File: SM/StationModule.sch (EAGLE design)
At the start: 25 parts, among them IC1 REG1117

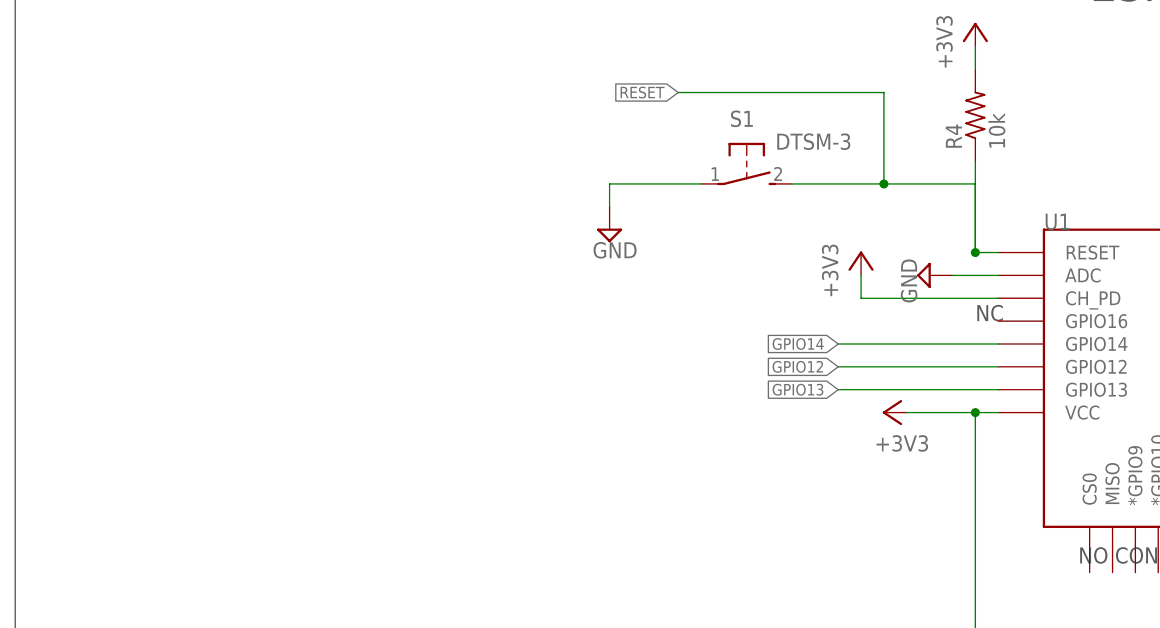
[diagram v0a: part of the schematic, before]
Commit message: silkscreen
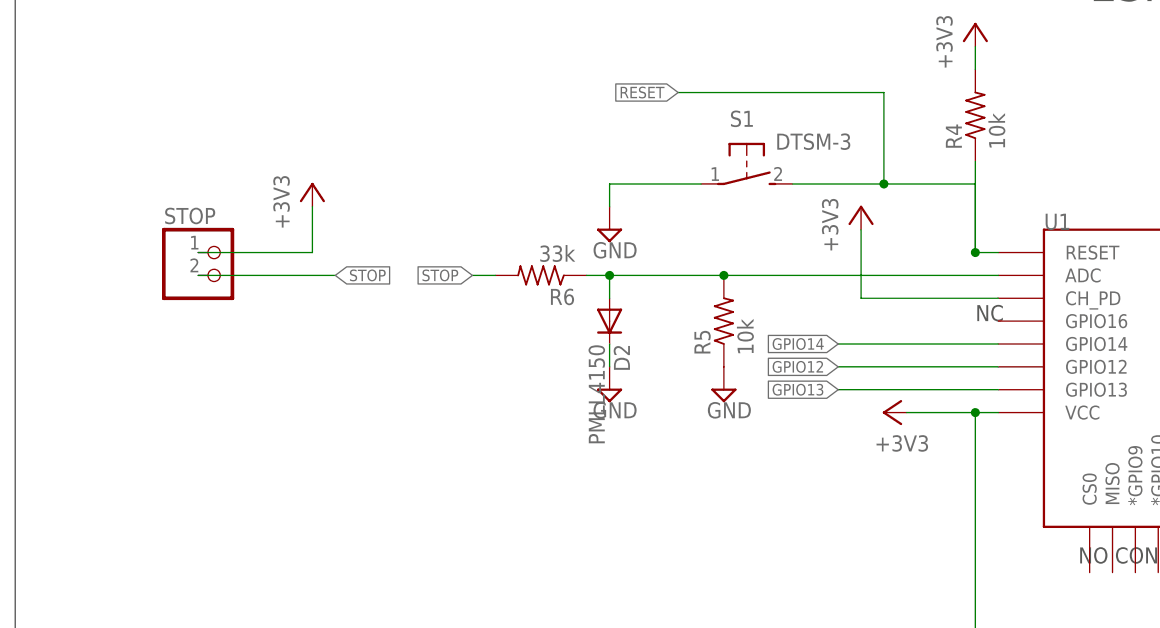
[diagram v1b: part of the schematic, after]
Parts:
- added D2: PMLL4150, diode:PMLL4150
- added R5: 10k, rcl:R-US_R0805
- added R6: 33k, rcl:R-US_R0805
- added STOP: (no value), pinhead+:PINHD-1X2
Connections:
- new net ADC: D2.A, R5.2, R6.1, U1.ADC
- new net STOP: R6.2, STOP.2
- net +3V3: now also STOP.1
- net GND: now also D2.C, R5.1; no longer U1.ADC
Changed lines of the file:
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@@
 <part name="SUPPLY14" library="supply2" deviceset="GND" device=""/>
 <part name="SUPPLY15" library="supply2" deviceset="GND" device=""/>
-<part name="SUPPLY16" library="supply2" deviceset="GND" device=""/>
 <part name="SPI_HEADER" library="pinhead+" deviceset="PINHD-1X5" device="" value="SPI-HEADER"/>
 <part name="SPI-HEADER" library="pinhead+" deviceset="PINHD-1X5" device="" value="SPI_HEADER"/>
@@
 <part name="H4" library="holes" deviceset="MOUNT-HOLE" device="3.0"/>
 <part name="USB" library="pinhead+" deviceset="PINHD-1X4" device="" value="USB-HEADER"/>
+<part name="STOP" library="pinhead+" deviceset="PINHD-1X2" device=""/>
+<part name="R5" library="rcl" deviceset="R-US_" device="R0805" value="10k"/>
+<part name="R6" library="rcl" deviceset="R-US_" device="R0805" value="33k"/>
+<part name="SUPPLY16" library="supply2" deviceset="GND" device=""/>
+<part name="SUPPLY18" library="supply2" deviceset="GND" device=""/>
+<part name="+3V9" library="supply1" deviceset="+3V3" device=""/>
+<part name="D2" library="diode" deviceset="PMLL4150" device=""/>
 </parts>
 <sheets>
@@
 <instance part="+3V3" gate="G$1" x="86.36" y="38.1"/>
 <instance part="+3V4" gate="G$1" x="121.92" y="35.56"/>
-<instance part="+3V5" gate="G$1" x="20.32" y="30.48"/>
+<instance part="+3V5" gate="G$1" x="20.32" y="35.56"/>
 <instance part="+3V6" gate="G$1" x="22.86" y="12.7" rot="R90"/>
 <instance part="SUPPLY4" gate="GND" x="-116.84" y="99.06"/>
@@
 <instance part="SUPPLY14" gate="GND" x="-38.1" y="86.36"/>
 <instance part="SUPPLY15" gate="GND" x="35.56" y="83.82"/>
-<instance part="SUPPLY16" gate="GND" x="27.94" y="27.94" rot="R270"/>
 <instance part="SPI_HEADER" gate="A" x="-111.76" y="-33.02"/>
 <instance part="SPI-HEADER" gate="A" x="-91.44" y="-33.02"/>
@@
 <instance part="H4" gate="G$1" x="119.38" y="-93.98"/>
 <instance part="USB" gate="A" x="-106.68" y="106.68"/>
+<instance part="STOP" gate="G$1" x="-50.8" y="27.94"/>
+<instance part="R5" gate="G$1" x="5.08" y="22.86" rot="R90"/>
+<instance part="R6" gate="G$1" x="-15.24" y="27.94" rot="R180"/>
+<instance part="SUPPLY16" gate="GND" x="-7.62" y="15.24"/>
+<instance part="SUPPLY18" gate="GND" x="5.08" y="15.24"/>
+<instance part="+3V9" gate="G$1" x="-40.64" y="38.1"/>
+<instance part="D2" gate="G$1" x="-7.62" y="22.86" rot="R270"/>
 </instances>
 <busses>
@@
 </segment>
 <segment>
-<pinref part="U1" gate="G$1" pin="ADC"/>
-<wire x1="35.56" y1="27.94" x2="30.48" y2="27.94" width="0.1524" layer="91"/>
-<pinref part="SUPPLY16" gate="GND" pin="GND"/>
-</segment>
-<segment>
 <pinref part="PROG-HEADER" gate="A" pin="6"/>
 <pinref part="SUPPLY17" gate="GND" pin="GND"/>
 <wire x1="-99.06" y1="63.5" x2="-121.92" y2="63.5" width="0.1524" layer="91"/>
+</segment>
+<segment>
+<pinref part="R5" gate="G$1" pin="1"/>
+<pinref part="SUPPLY18" gate="GND" pin="GND"/>
+</segment>
+<segment>
+<pinref part="SUPPLY16" gate="GND" pin="GND"/>
+<pinref part="D2" gate="G$1" pin="C"/>
+<wire x1="-7.62" y1="20.32" x2="-7.62" y2="17.78" width="0.1524" layer="91"/>
 </segment>
 </net>
@@
 <pinref part="U1" gate="G$1" pin="CH_PD"/>
 <wire x1="35.56" y1="25.4" x2="20.32" y2="25.4" width="0.1524" layer="91"/>
-<wire x1="20.32" y1="25.4" x2="20.32" y2="27.94" width="0.1524" layer="91"/>
+<wire x1="20.32" y1="25.4" x2="20.32" y2="33.02" width="0.1524" layer="91"/>
 <pinref part="+3V5" gate="G$1" pin="+3V3"/>
 </segment>
@@
 <wire x1="-99.06" y1="73.66" x2="-121.92" y2="73.66" width="0.1524" layer="91"/>
 </segment>
+<segment>
+<pinref part="STOP" gate="G$1" pin="1"/>
+<wire x1="-53.34" y1="30.48" x2="-40.64" y2="30.48" width="0.1524" layer="91"/>
+<pinref part="+3V9" gate="G$1" pin="+3V3"/>
+<wire x1="-40.64" y1="35.56" x2="-40.64" y2="30.48" width="0.1524" layer="91"/>
+</segment>
 </net>
 <net name="+5V" class="0">
@@
 </segment>
 </net>
+<net name="STOP" class="0">
+<segment>
+<pinref part="STOP" gate="G$1" pin="2"/>
+<wire x1="-53.34" y1="27.94" x2="-38.1" y2="27.94" width="0.1524" layer="91"/>
+<label x="-38.1" y="27.94" size="1.27" layer="95" xref="yes"/>
+</segment>
+<segment>
+<pinref part="R6" gate="G$1" pin="2"/>
+<wire x1="-20.32" y1="27.94" x2="-22.86" y2="27.94" width="0.1524" layer="91"/>
+<label x="-22.86" y="27.94" size="1.27" layer="95" rot="R180" xref="yes"/>
+</segment>
+</net>
+<net name="ADC" class="0">
+<segment>
+<pinref part="U1" gate="G$1" pin="ADC"/>
+<wire x1="35.56" y1="27.94" x2="5.08" y2="27.94" width="0.1524" layer="91"/>
+<pinref part="R5" gate="G$1" pin="2"/>
+<wire x1="5.08" y1="27.94" x2="-7.62" y2="27.94" width="0.1524" layer="91"/>
+<junction x="5.08" y="27.94"/>
+<pinref part="R6" gate="G$1" pin="1"/>
+<wire x1="-7.62" y1="27.94" x2="-10.16" y2="27.94" width="0.1524" layer="91"/>
+<wire x1="-7.62" y1="25.4" x2="-7.62" y2="27.94" width="0.1524" layer="91"/>
+<junction x="-7.62" y="27.94"/>
+<pinref part="D2" gate="G$1" pin="A"/>
+</segment>
+</net>
